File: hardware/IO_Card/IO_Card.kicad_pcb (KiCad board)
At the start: 2 copper layers, 100 x 99.9 mm, 18 parts, among them J1 6502 Edge, J2 6502 Pinheader, J3 Port A, J4 Port B, J7 Port A, J8 Port B, J9 VIA IO Select, U1 W65C22NxP, U2 W65C22NxP

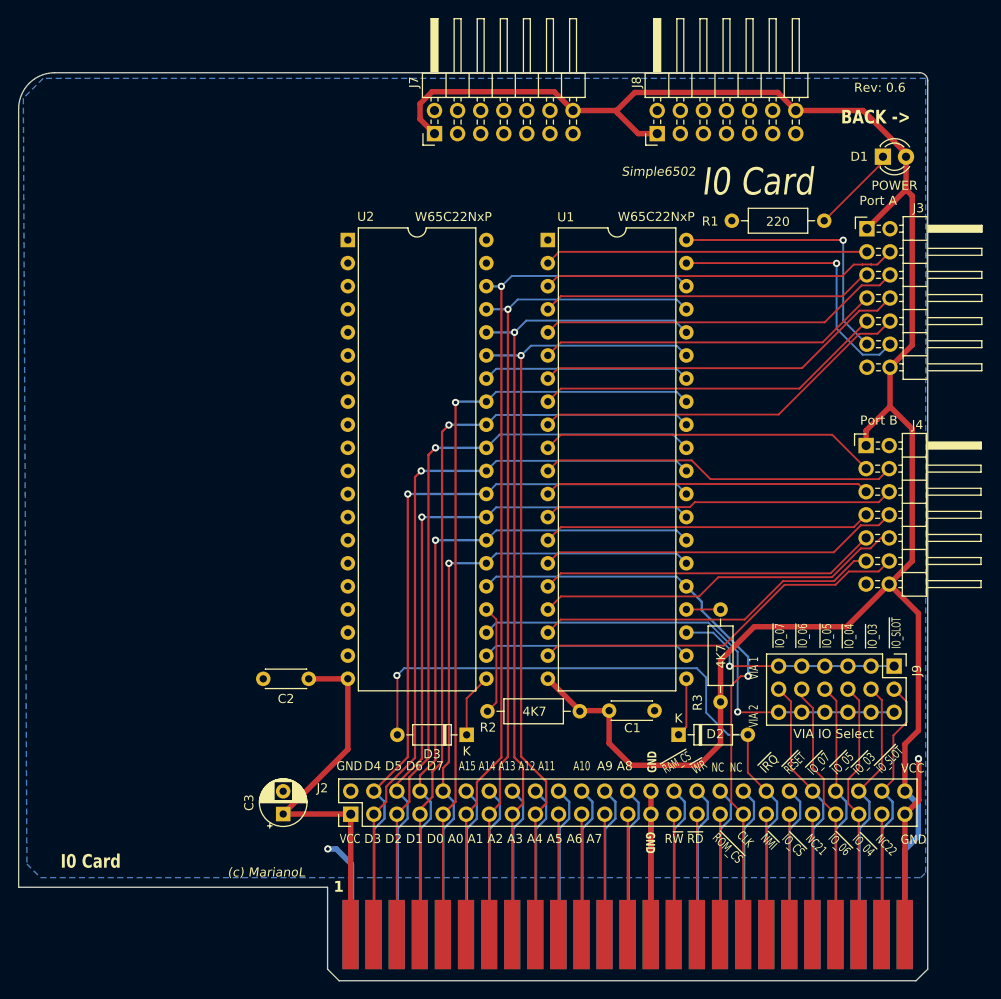
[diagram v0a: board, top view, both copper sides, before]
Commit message: IO Card is Rev 1.0 PCB complete
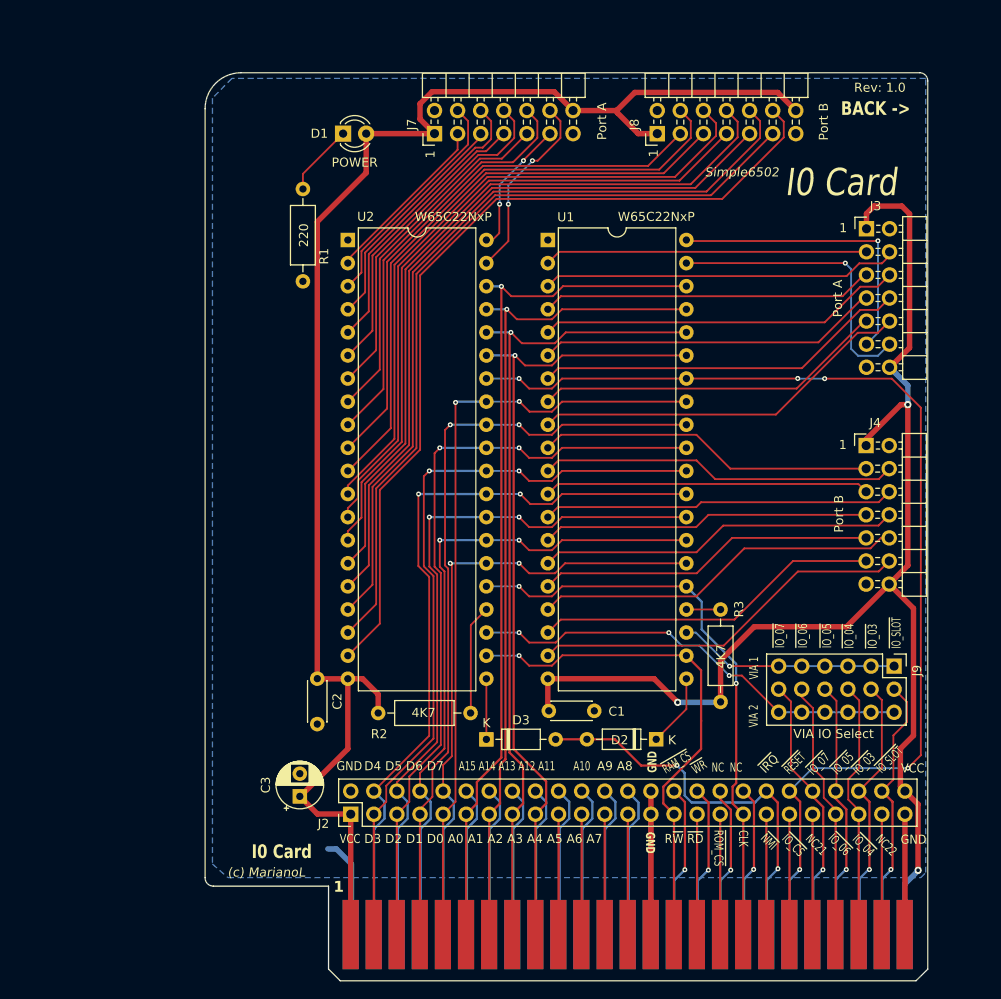
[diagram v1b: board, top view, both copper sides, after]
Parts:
- J3, J4, J7, J8: footprint Connector_PinHeader_2.54mm:PinHeader_2x07_P2.54mm_Horizontal -> Connector_PinHeader_2.54mm:PinHeader_2x07_P2.54mm_Horizontal_Edge
- moved D1 59.4 mm to (55.5, 37.3)
- moved R1 57.4 mm to (51.1, 43.4), turned to -90 degrees
- moved C1 6.63 mm to (78.1, 100.8)
- moved C3 2.67 mm to (50.7, 110.2)
- moved D2 2.51 mm to (89.9, 103.9), turned to 180 degrees
- moved D3 2.23 mm to (71.2, 103.9), turned to 0 degrees
- moved R2 1.87 mm to (69.5, 101.0), turned to 180 degrees
- moved C2 0.94 mm to (52.6, 97.2), turned to -90 degrees
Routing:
- net /2CB2: track 0.00 -> 94.9 mm
- net /2CB1: track 0.00 -> 88.2 mm
- net /2PB7: track 0.00 -> 87.9 mm
- net /~{RESET}: track 39.7 -> 121.1 mm, vias 0 -> 5
- net /2PB6: track 0.00 -> 81.2 mm
- net /2PB5: track 0.00 -> 81.0 mm
- net /2PB4: track 0.00 -> 74.3 mm
- net /2PB3: track 0.00 -> 74.2 mm
- net /2PB2: track 0.00 -> 67.3 mm
- net /2PB1: track 0.00 -> 67.0 mm
- net /2PB0: track 0.00 -> 60.3 mm
- net /2PA7: track 0.00 -> 45.7 mm
- net VCC: track 272.1 -> 317.2 mm, vias 0 -> 3
- net /2PA6: track 0.00 -> 39.1 mm
- net /2PA5: track 0.00 -> 38.8 mm
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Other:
- board size 100 x 99.9 mm -> 79.5 x 99.9 mm
